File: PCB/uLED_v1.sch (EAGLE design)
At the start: 9 parts, among them IC1 ATSAMD21E

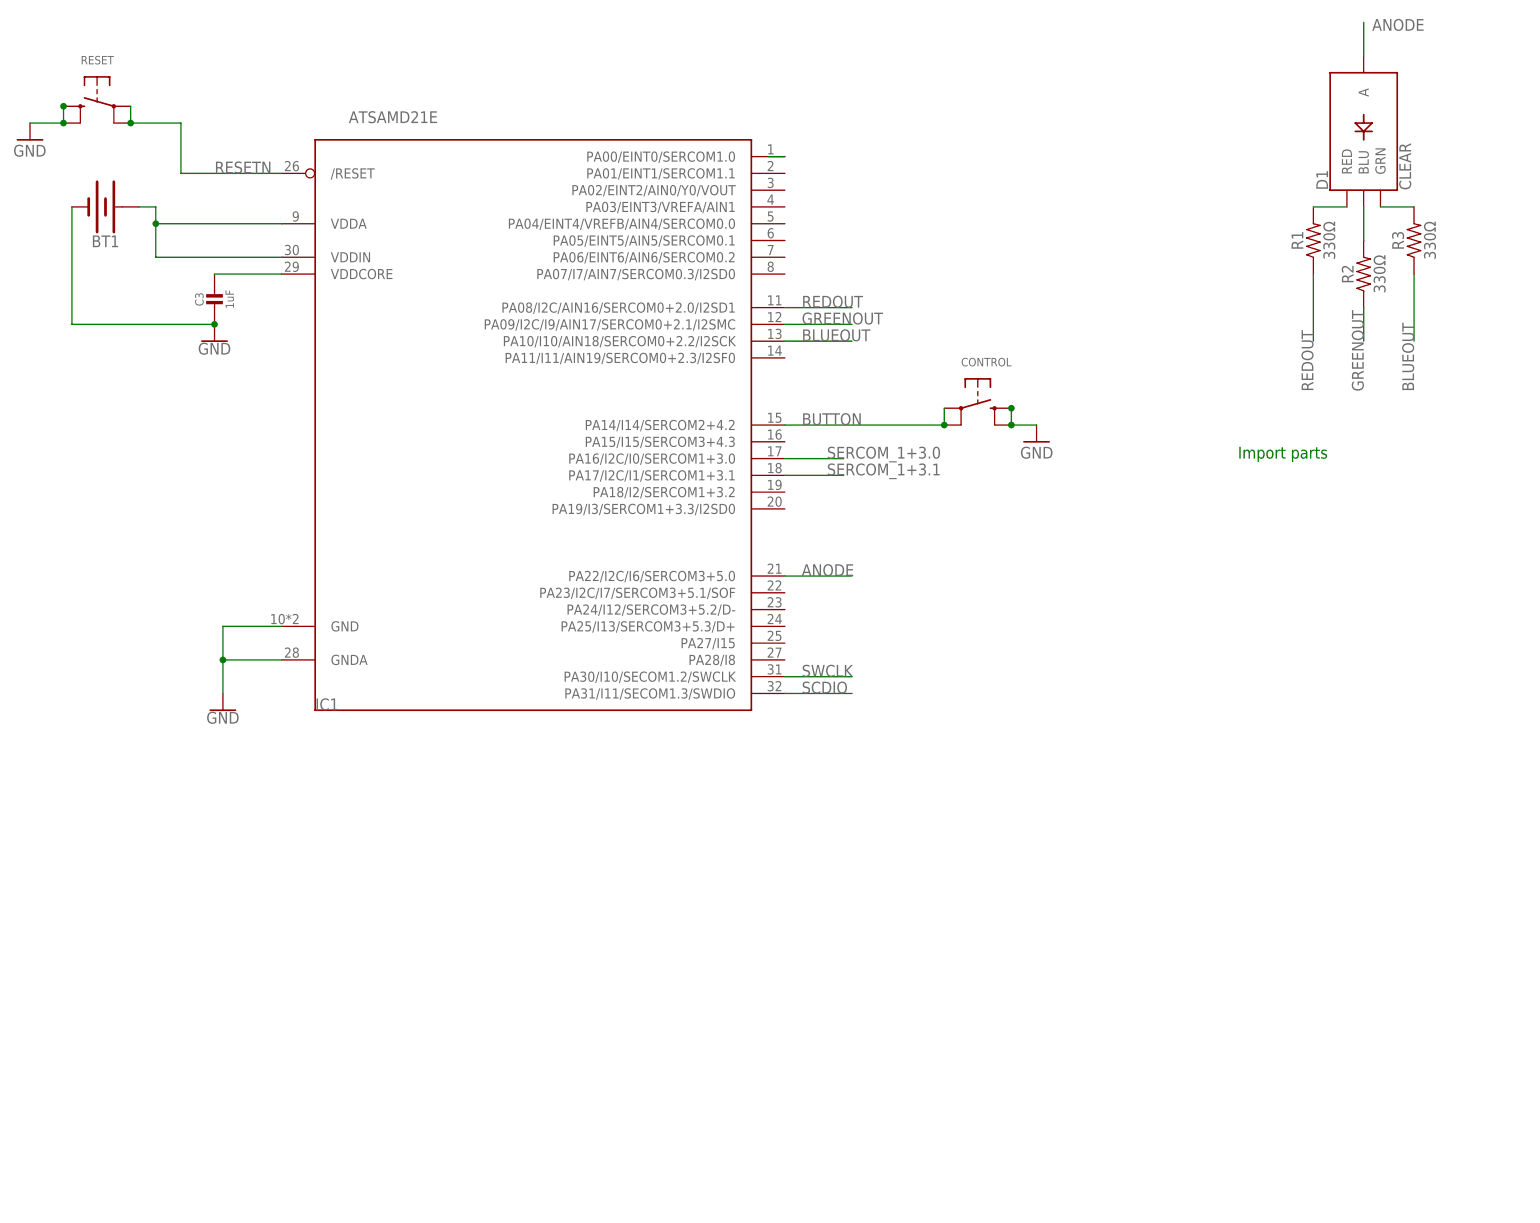
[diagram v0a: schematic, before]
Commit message: PBG in progress
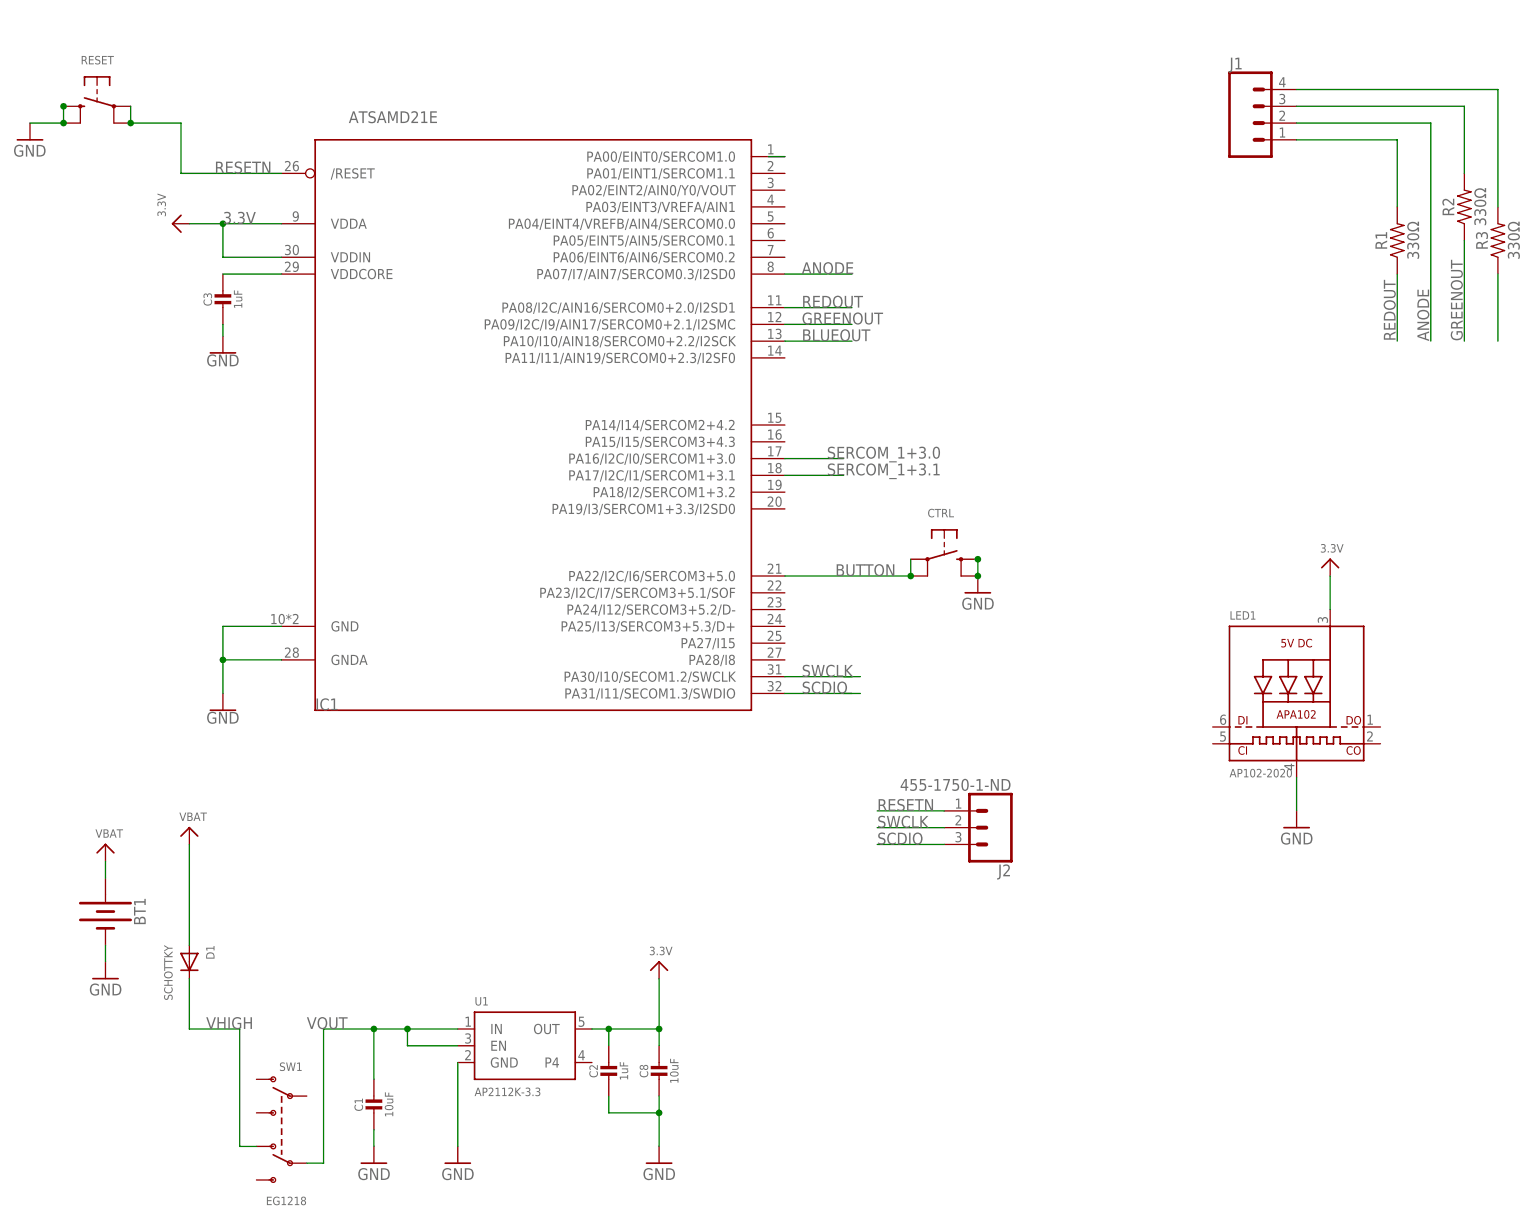
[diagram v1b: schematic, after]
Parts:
- removed CONTROL: (no value), microbuilder:SWITCH_TACT_SMT4.6X2.8
- added C1, C8: 10uF, microbuilder:CAP_CERAMIC0805-NOOUTLINE
- added C2: 1uF, microbuilder:CAP_CERAMIC0603_NO
- added CTRL: (no value), microbuilder:SWITCH_TACT_SMT4.6X2.8
- added J1: (no value), SparkFun-Connectors:CONN_04
- added J2: 455-1750-1-ND, SparkFun-Connectors:CONN_03
- added LED1: AP102-2020, microbuilder:APA1022020
- added SW1: EG1218, microbuilder:SWITCH_DPDTEG1390
- added U1: AP2112K-3.3, microbuilder:VREG_SOT23-5
- D1: value CLEAR -> SCHOTTKY; device SparkFun-LED:LED-RGB-CACLEAR -> adafruit:DIODE_SOD-123FL
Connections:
- removed net N$4: BT1.+, IC1.VDDA, IC1.VDDIN
- new net 3.3V: C2.1, C8.1, IC1.VDDA, IC1.VDDIN, LED1.VDD, U1.OUT
- new net VBAT: BT1.+, D1.A
- new net VHIGH: D1.C, SW1.O2
- new net VOUT: C1.1, SW1.P2, U1.EN, U1.IN
- net ANODE: now also IC1.PA07/I7/AIN7/SERCOM0.3/I2SD0, J1.2; no longer D1.A, IC1.PA22/I2C/I6/SERCOM3+5.0
- net BUTTON: now also CTRL.P, CTRL.P1, IC1.PA22/I2C/I6/SERCOM3+5.0; no longer CONTROL.P, CONTROL.P1, IC1.PA14/I14/SERCOM2+4.2
- net GND: now also C1.2, C2.2, C8.2, CTRL.S, CTRL.S1, LED1.GND, U1.GND; no longer CONTROL.S, CONTROL.S1
- net N$1: now also J1.1; no longer D1.RED
- net N$2: now also J1.4; no longer D1.GRN
- net N$3: now also J1.3; no longer D1.BLU
- net RESETN: now also J2.1
- net SCDIO: now also J2.3
- net SWCLK: now also J2.2
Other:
- note removed: "Import parts"
- moved on the sheet: BT1, C3, R1, R2, R3
